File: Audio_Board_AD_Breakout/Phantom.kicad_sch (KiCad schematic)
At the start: 35 parts, among them IC3 TPS73250DBVR, IC4 TPS73250DBVR, J1 SBH11-PBPC-D10-ST-BK, J11 PINHD_1x1_Male, J13 PINHD_1x10_Female, J14 PINHD_1x10_Female, J8 PINHD_1x5_Female

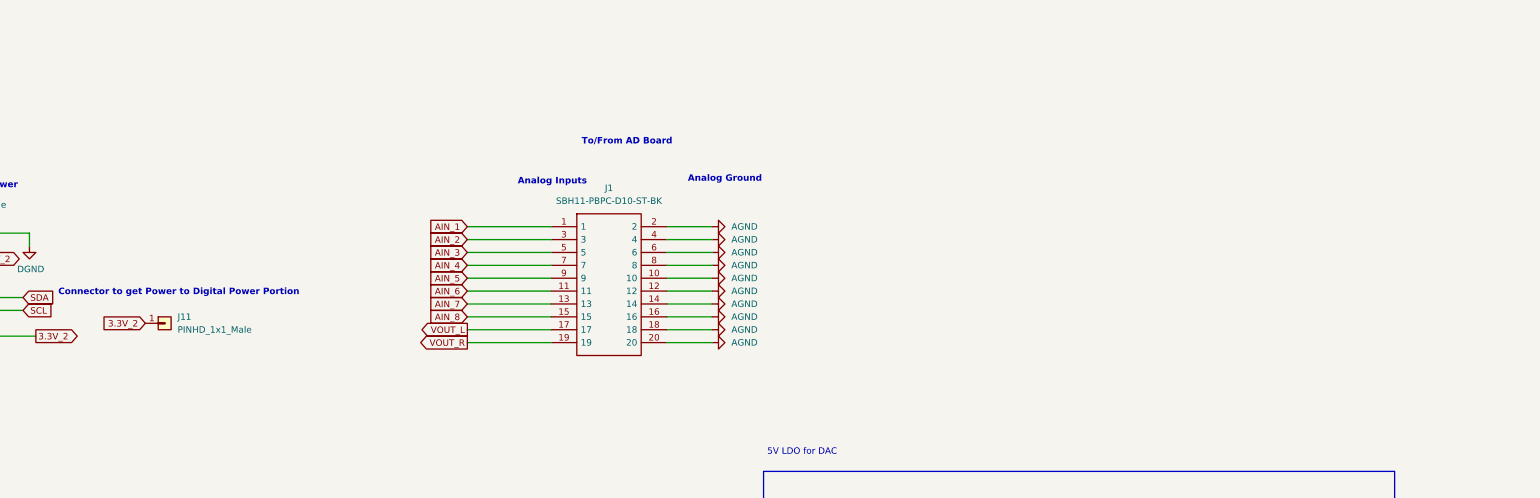
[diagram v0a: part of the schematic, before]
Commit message: aaaah (cooked)
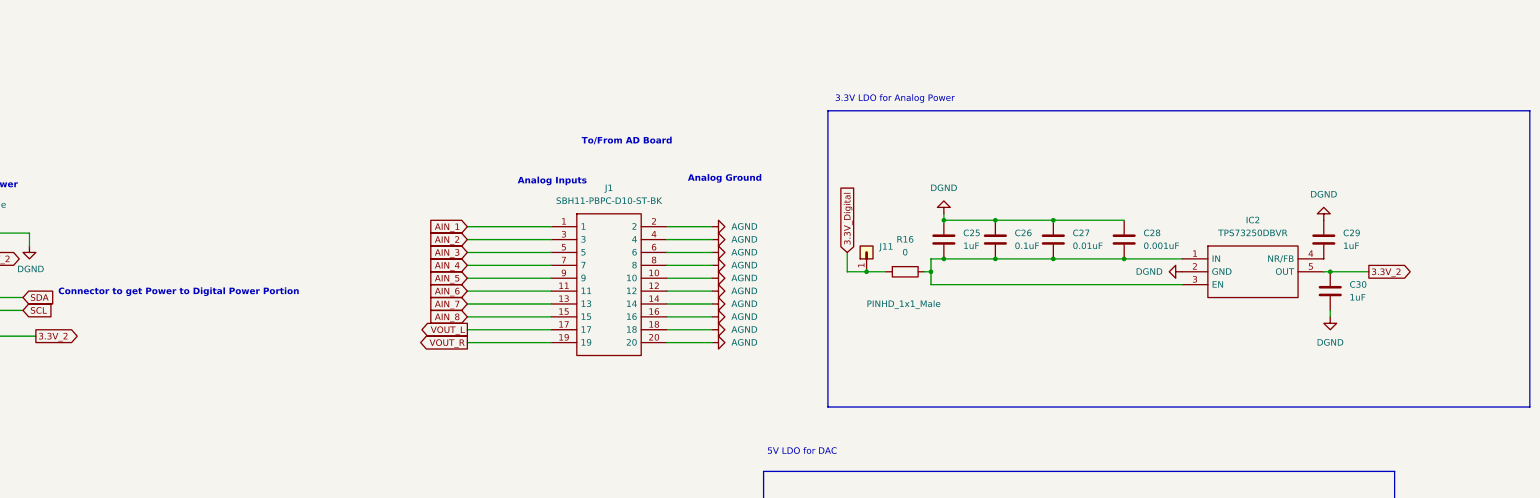
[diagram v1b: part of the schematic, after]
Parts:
- added C25, C29, C30: 1uF, Capacitor_SMD:C_0402_1005Metric, symbol Device:C
- added C26: 0.1uF, Capacitor_SMD:C_0402_1005Metric, symbol Device:C
- added C27: 0.01uF, Capacitor_SMD:C_0402_1005Metric, symbol Device:C
- added C28: 0.001uF, Capacitor_SMD:C_0402_1005Metric, symbol Device:C
- added IC2: TPS73250DBVR, SOT95P280X145-5N, symbol SamacSys_Parts:TPS73250DBVR
- added R16: 0, Resistor_SMD:R_0805_2012Metric, symbol Device:R
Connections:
- net 3.3V_2: now also C30.1, IC2.5 (OUT); no longer J11.1
- net DGND: now also C25.1, C26.1, C27.1, C28.1, C29.1, C30.2, IC2.2 (GND)
- new net: C25.2, C26.2, C27.2, C28.2, IC2.1 (IN), IC2.3 (EN), R16.1
- new net: C29.2, IC2.4 (NR/FB)
- new net 3.3V_Digital: J11.1, R16.2
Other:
- moved on the sheet: J11
